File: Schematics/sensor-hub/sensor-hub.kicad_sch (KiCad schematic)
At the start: 1 part

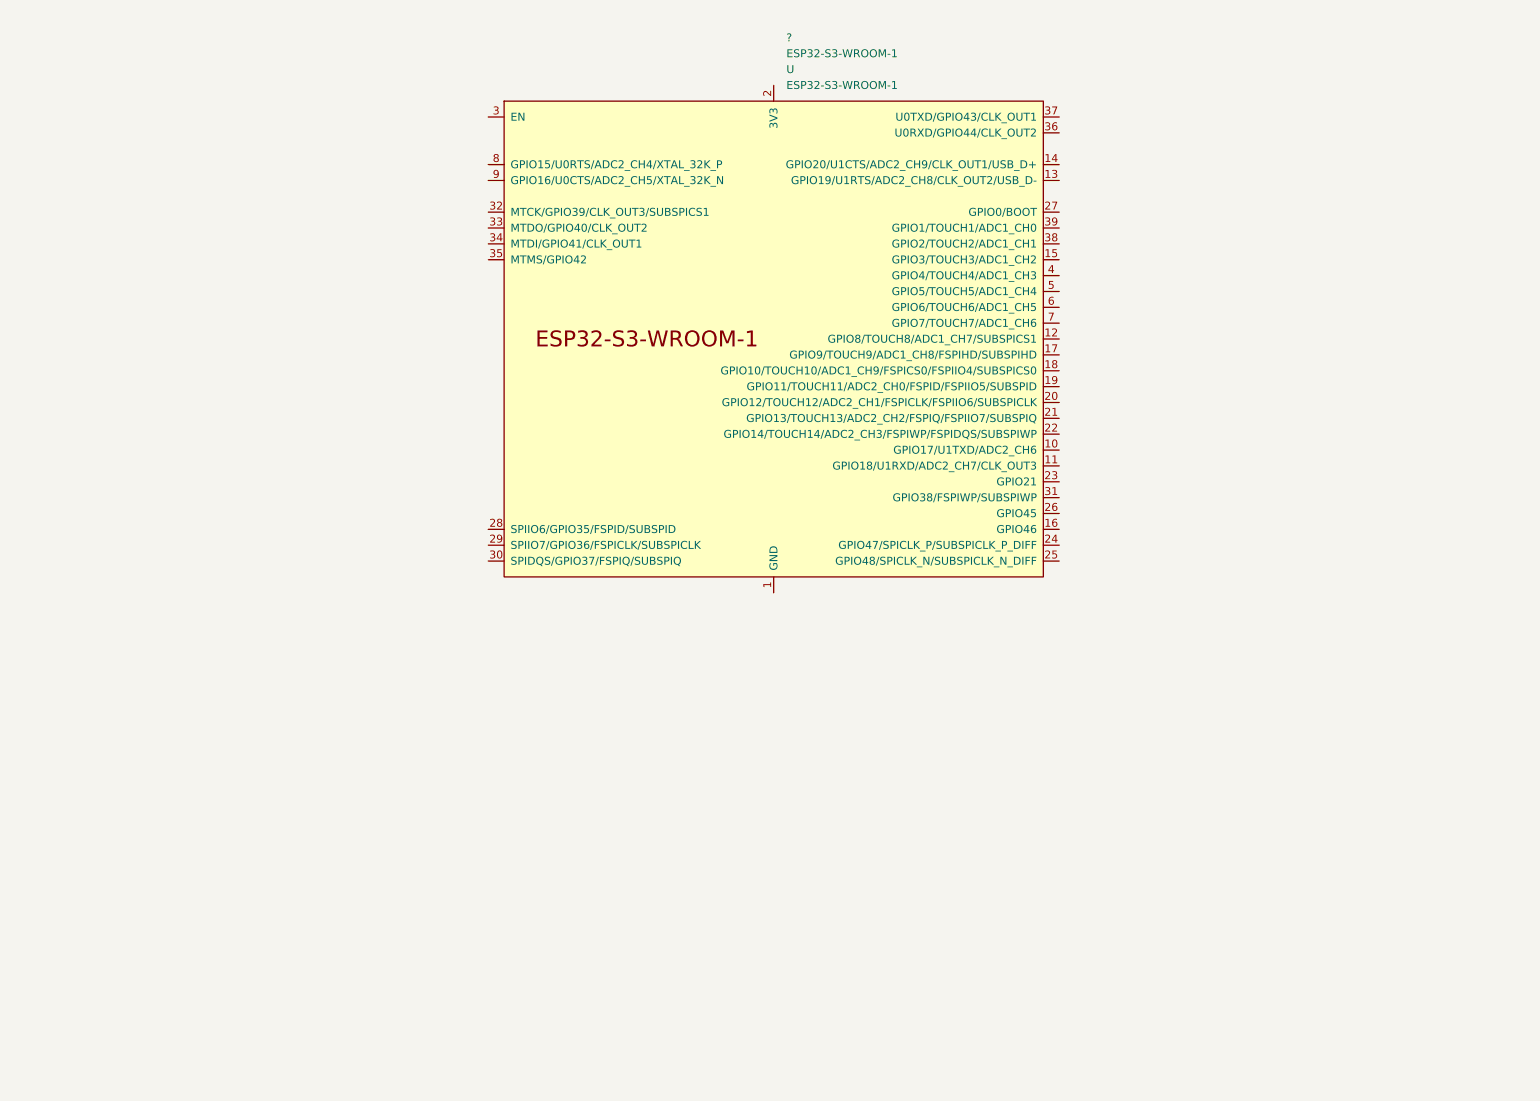
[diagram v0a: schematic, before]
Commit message: managers meeting schematics
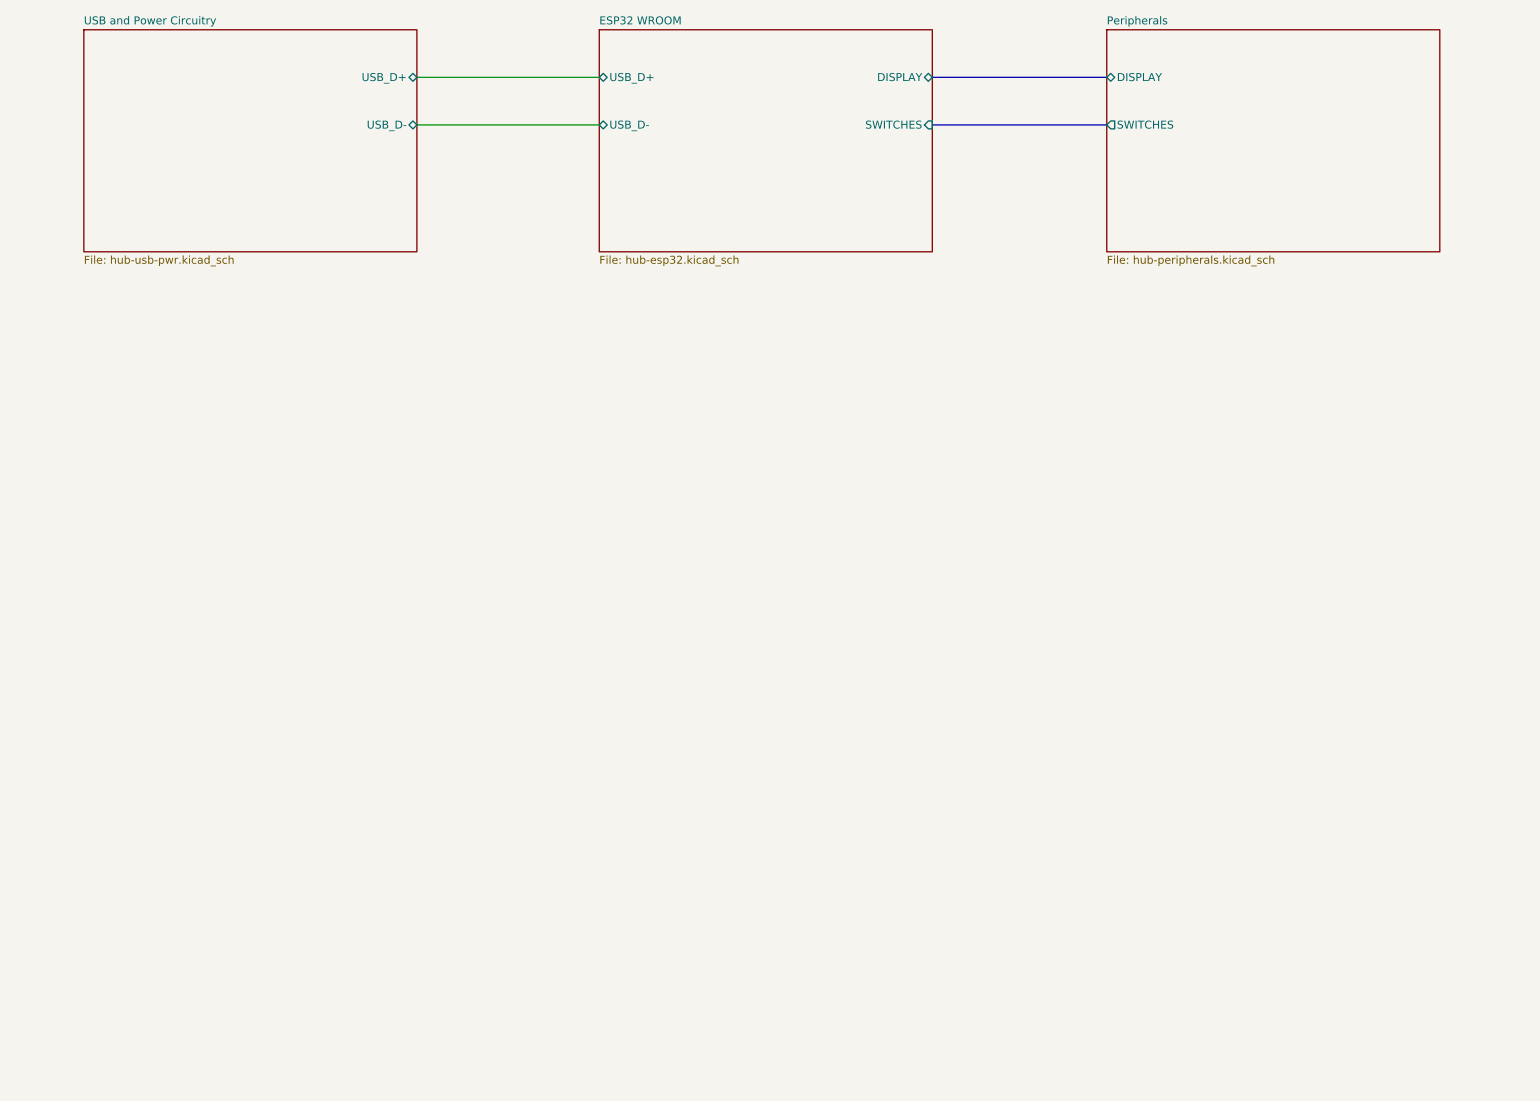
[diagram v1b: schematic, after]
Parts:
- removed ?: ESP32-S3-WROOM-1, symbol Espressif:ESP32-S3-WROOM-1
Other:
- added sheet ESP32 WROOM (hub-esp32.kicad_sch)
- added sheet Peripherals (hub-peripherals.kicad_sch)
- added sheet USB and Power Circuitry (hub-usb-pwr.kicad_sch)

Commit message: schematic and pcb upload
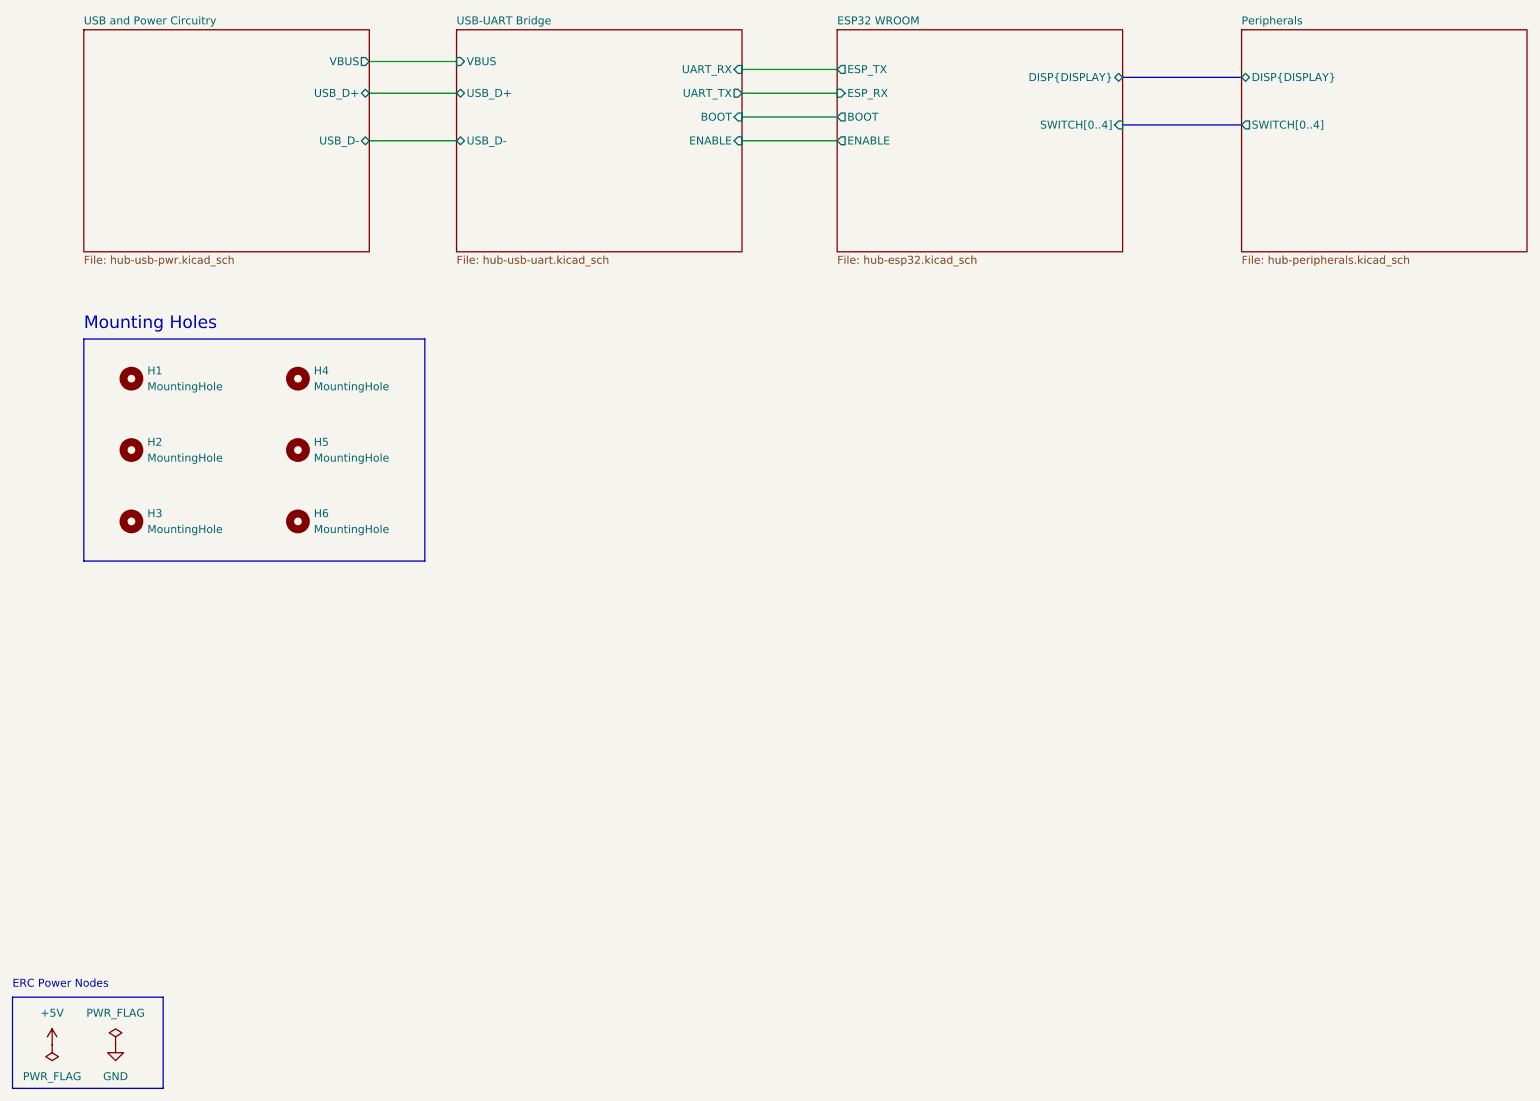
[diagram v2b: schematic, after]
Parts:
- added H1, H2, H3, H4, H5, H6: MountingHole, MountingHole:MountingHole_3.2mm_M3, symbol Mechanical:MountingHole
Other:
- added sheet USB-UART Bridge (hub-usb-uart.kicad_sch)
- sheet ESP32 WROOM ports: added BOOT, DISP{DISPLAY}, ENABLE, ESP_RX, ESP_TX, SWITCH[0..4]; removed DISPLAY, SWITCHES, USB_D+, USB_D-
- sheet Peripherals ports: added DISP{DISPLAY}, SWITCH[0..4]; removed DISPLAY, SWITCHES
- sheet USB and Power Circuitry ports: added VBUS; removed none
- note added: "ERC Power Nodes"
- note added: "Mounting Holes"
